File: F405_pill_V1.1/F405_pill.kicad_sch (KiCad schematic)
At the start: 50 parts, among them J1 Conn_01x04_Male, J2 Conn_01x04_Male, J4 TYPE-C-31-M-12, U1 STM32F405RGTx, U2 MAX3051EKA+T, U3 LM1117-3.3, U4 STM32F405_pill, U5 HT7550-1, Y1 Crystal_GND24

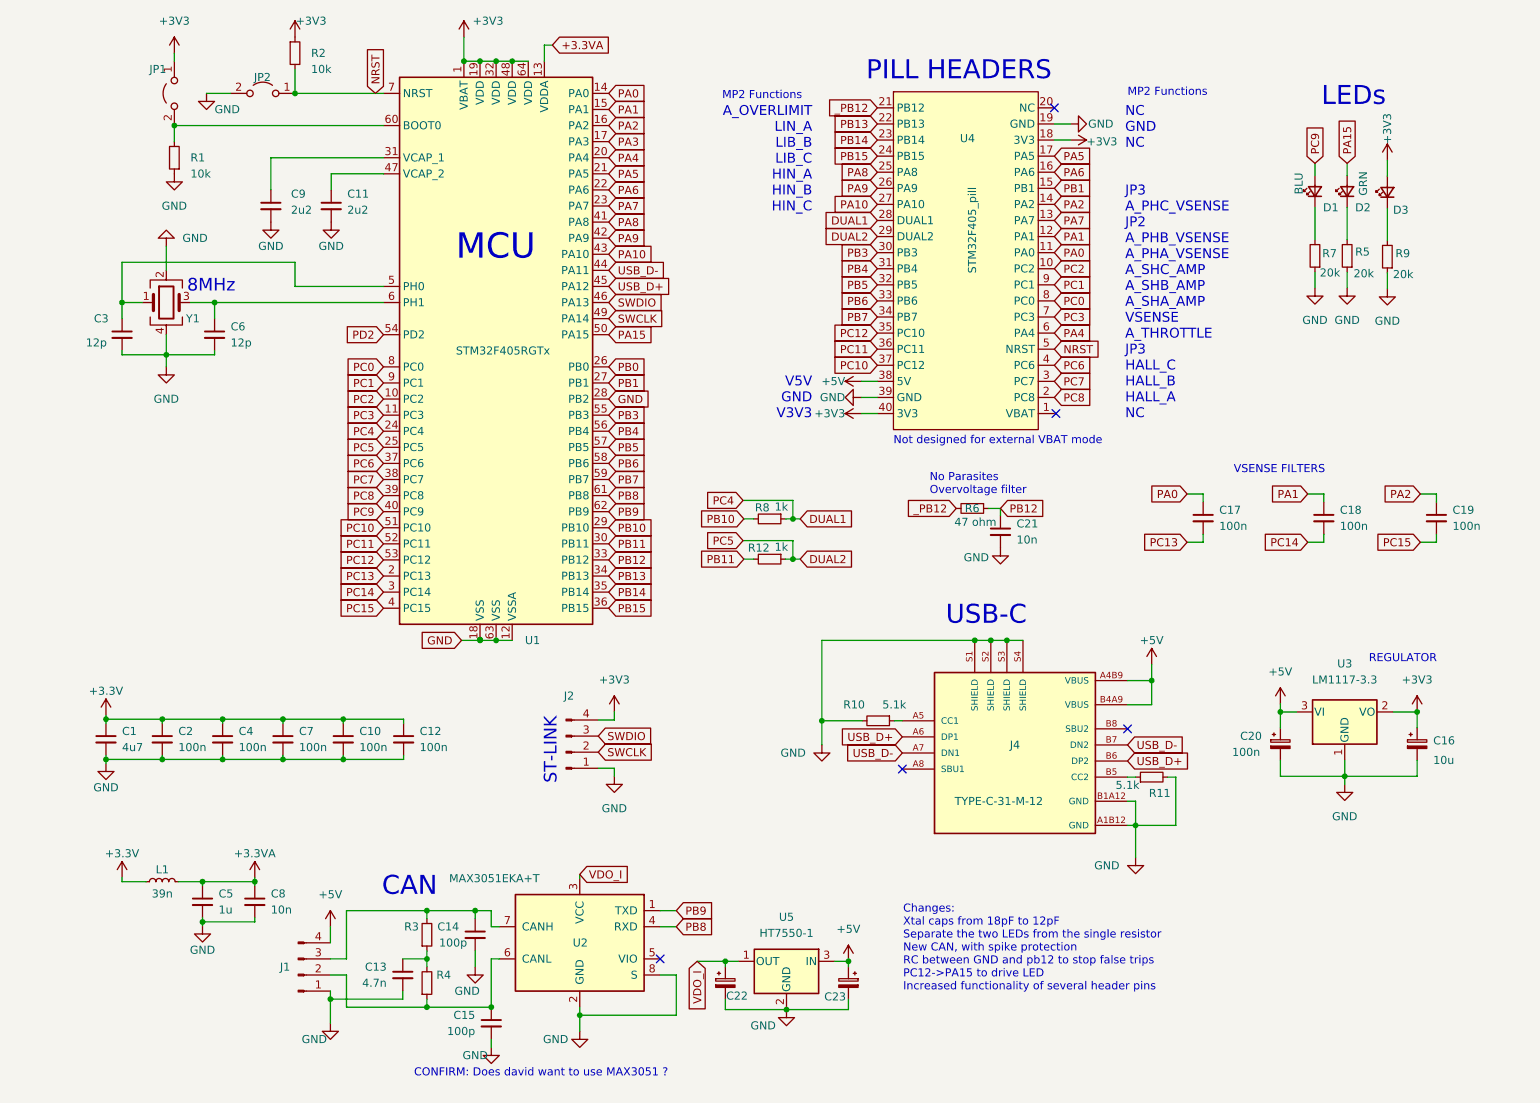
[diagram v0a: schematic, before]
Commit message: finalizing
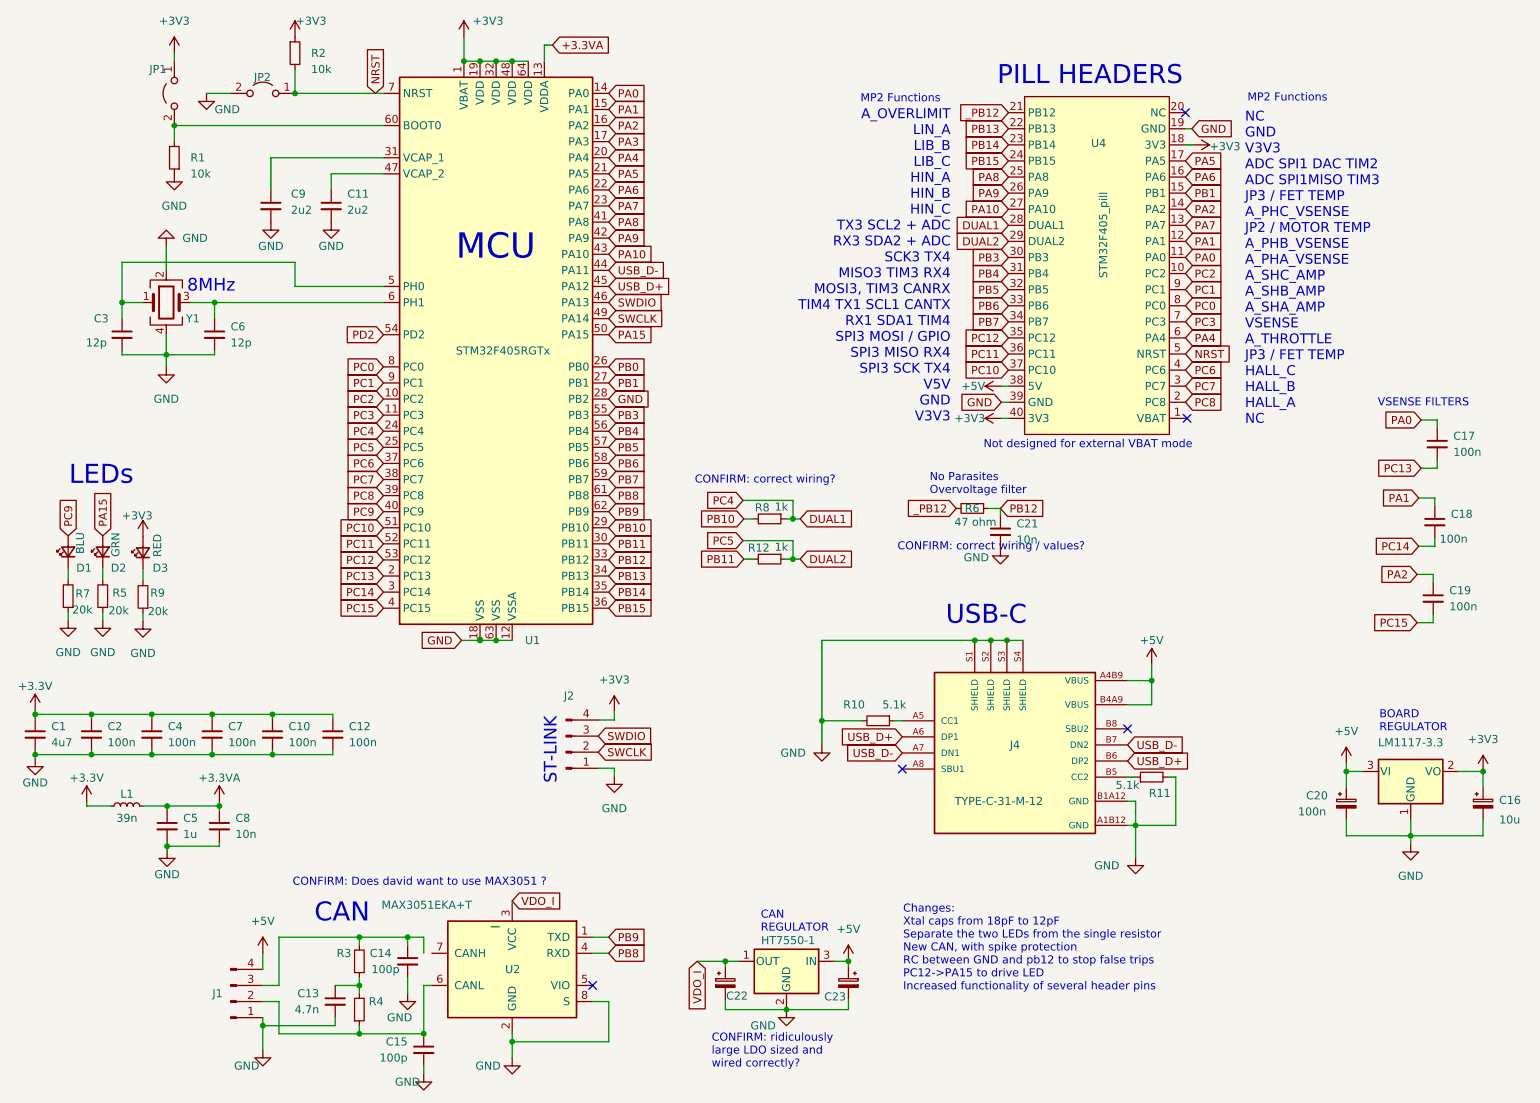
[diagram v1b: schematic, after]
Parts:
- D3: value RED_LED -> RED
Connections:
- net at C14.1, J1.3 (Pin_3), R3.2: no longer U2.7 (CANH)
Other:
- note added: "A_OVERLIMIT LIN_A LIB_B LIB_C HIN_A HIN_B HIN_C TX3 SCL2 + ADC RX3 SDA2 + ADC SCK3 TX4 MISO3 TIM3 RX4 MOSI3, TIM3 CANRX TIM4 TX1 SCL1 CANTX RX1 SDA1 TIM4 SPI3 MOSI / GPIO SPI3 MISO RX4 SPI3 SCK TX4 V5V GND V3V3"
- note added: "BOARD REGULATOR"
- note added: "CAN REGULATOR"
- note added: "CONFIRM: correct wiring / values?"
- note added: "CONFIRM: correct wiring?"
- note added: "CONFIRM: ridiculously large LDO sized and wired correctly?"
- note added: "NC GND V3V3 ADC SPI1 DAC TIM2 ADC SPI1MISO TIM3 JP3 / FET TEMP A_PHC_VSENSE JP2 / MOTOR TEMP A_PHB_VSENSE A_PHA_VSENSE A_SHC_AMP A_SHB_AMP A_SHA_AMP VSENSE A_THROTTLE JP3 / FET TEMP HALL_C HALL_B HALL_A NC"
- note removed: "A_OVERLIMIT LIN_A LIB_B LIB_C HIN_A HIN_B HIN_C V5V GND V3V3"
- note removed: "NC GND NC JP3 A_PHC_VSENSE JP2 A_PHB_VSENSE A_PHA_VSENSE A_SHC_AMP A_SHB_AMP A_SHA_AMP VSENSE A_THROTTLE JP3 HALL_C HALL_B HALL_A NC"
- note removed: "REGULATOR"
- moved on the sheet: C1, C10, C12, C13, C14, C15, C16, C17, C18, C19, C2, C20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
